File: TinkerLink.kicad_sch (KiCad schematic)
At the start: 26 parts, among them J1 Conn_01x06_Pin, Q1 IRF4905S, Q2 MMBT2222A, SW1 TS-061D-250D4-P, U1 ESP-01F-2M, U2 ME6211C33M5, U3 AP63203WU

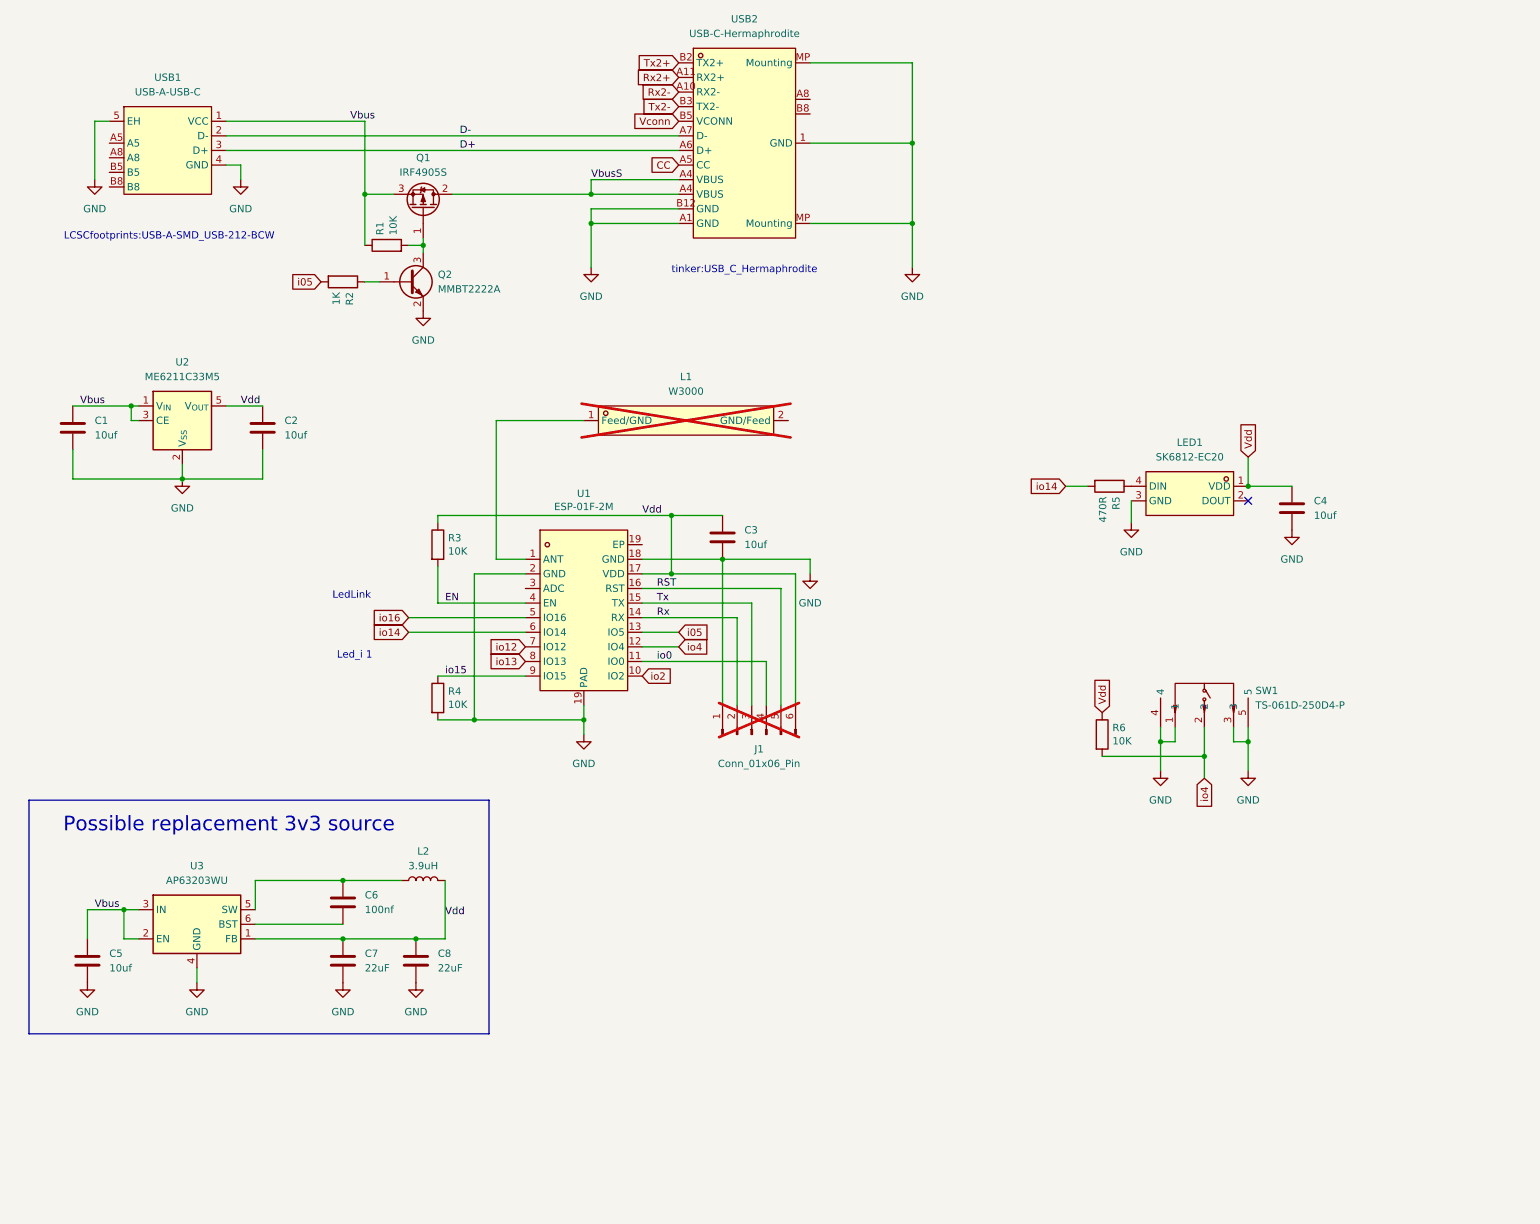
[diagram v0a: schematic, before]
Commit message: new 3v3 in place(ish)
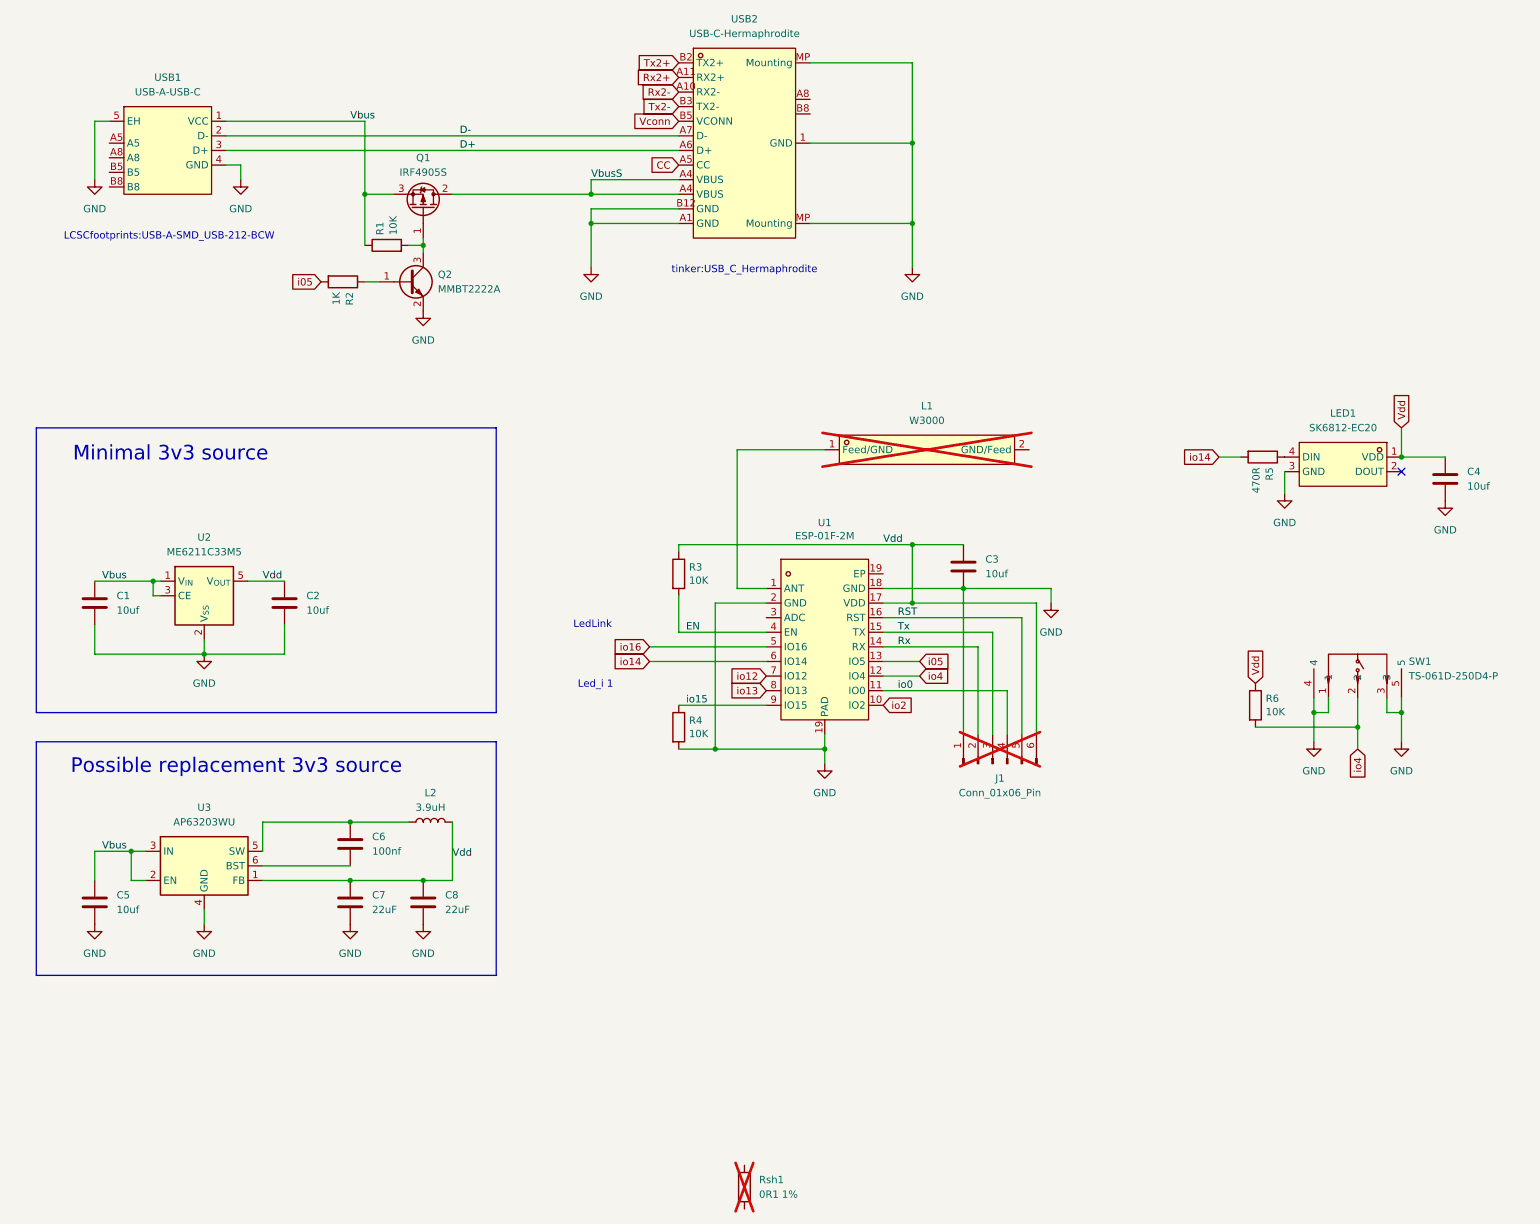
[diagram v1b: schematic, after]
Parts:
- added Rsh1: 0R1 1%, Resistor_SMD:R_2512_6332Metric, symbol Device:R
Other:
- note added: "Minimal 3v3 source"
- moved on the sheet: C1, C2, C3, C4, C5, C6, C7, C8, J1, L1, L2, LED1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
